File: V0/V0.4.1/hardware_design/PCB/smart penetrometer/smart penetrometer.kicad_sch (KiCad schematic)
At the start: 22 parts, among them J1 Conn_01x02_Female, J2 XLR3_Switched, J3 Conn_01x07_Female, U1 ADS1120-PW, U2 DS3231M, U3 4023, U4 ADS1115IDGS

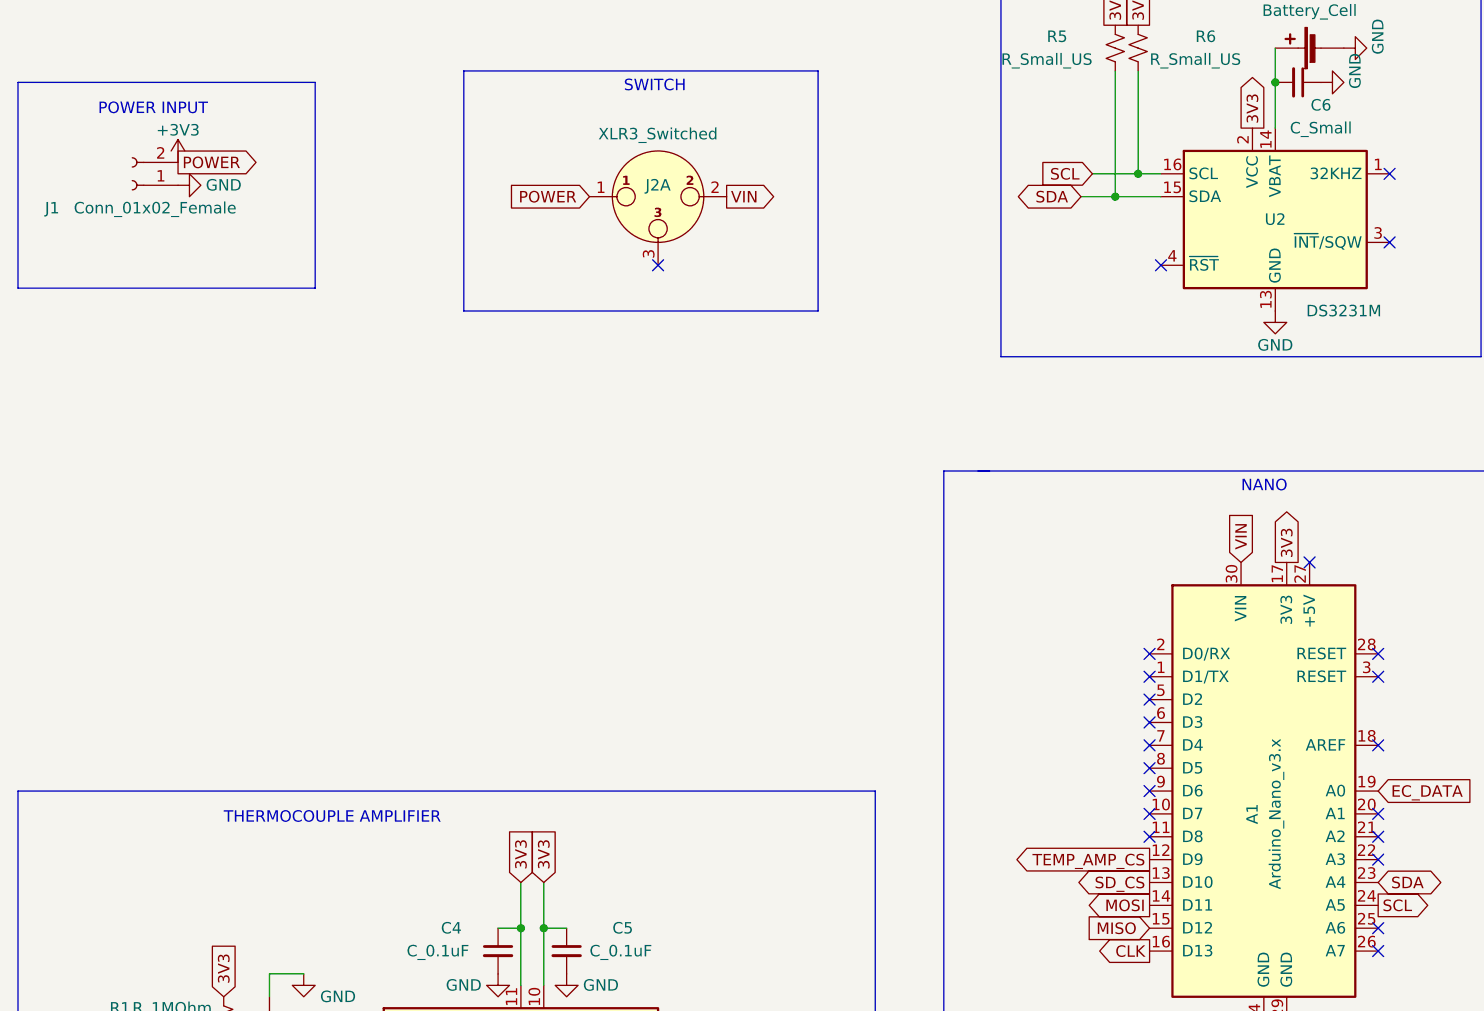
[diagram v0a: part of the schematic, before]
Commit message: PCB V0.4.1 UPDATE
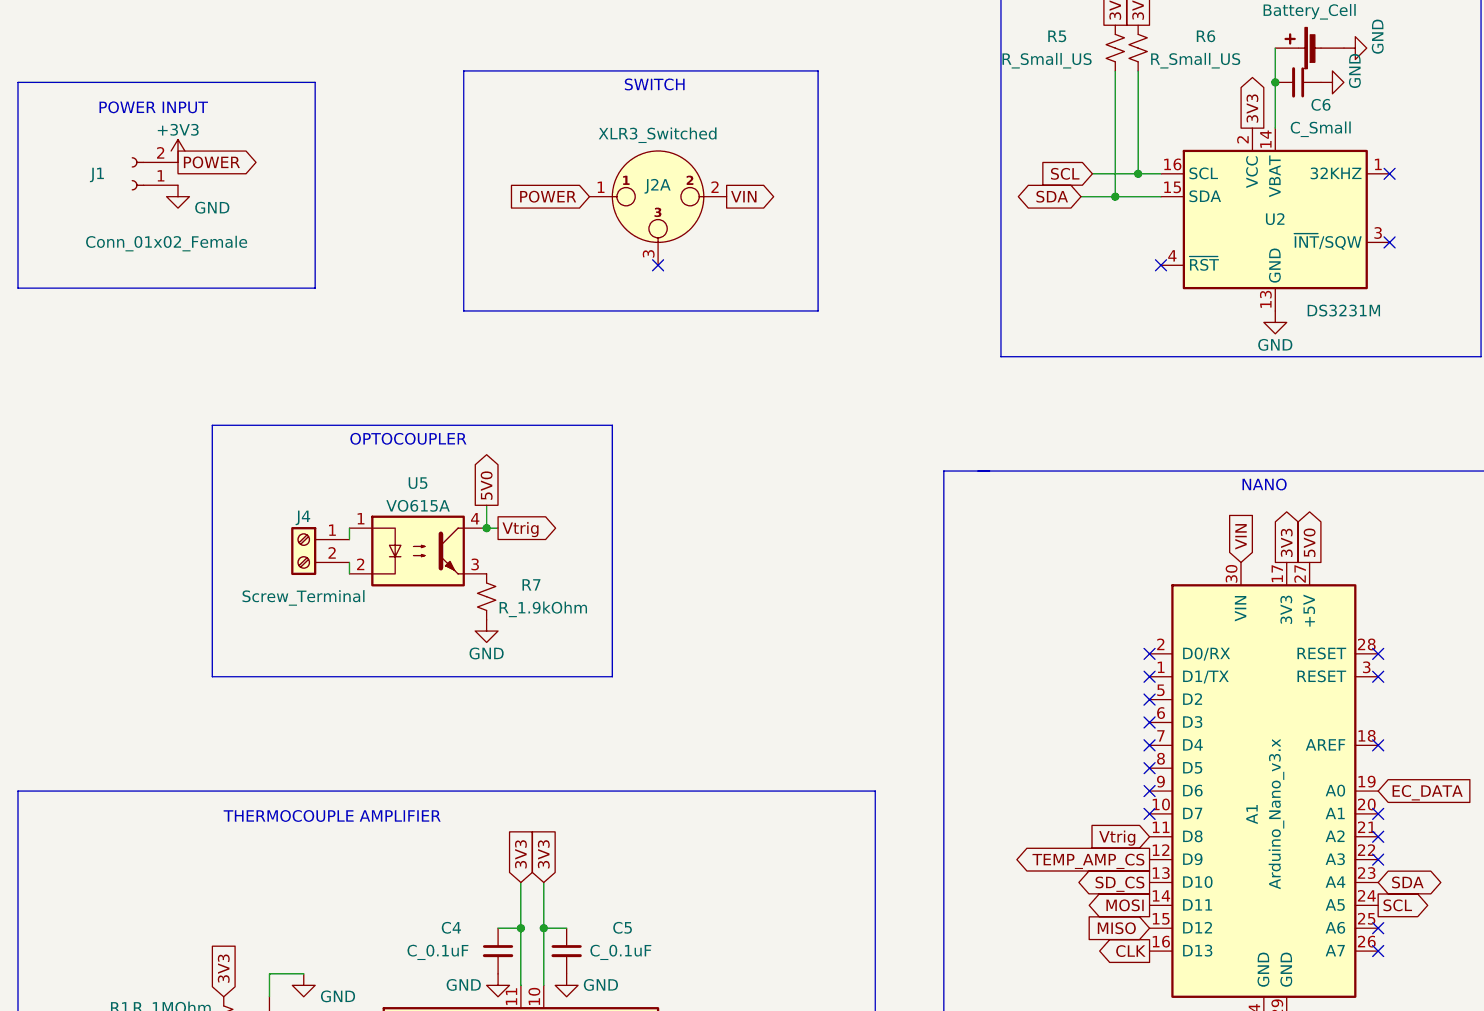
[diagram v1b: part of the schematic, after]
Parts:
- added J4: Screw_Terminal, TerminalBlock:TerminalBlock_bornier-2_P5.08mm, symbol Connector:Screw_Terminal_01x02
- added R7: R_1.9kOhm, Resistor_SMD:R_1206_3216Metric, symbol Device:R_Small_US
- added U5: VO615A, footprints:Vishay_VOS615A, symbol Isolator:VO615A
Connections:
- net GND: now also R7.2
- net 5V0: now reaches A1.11 (D8)
- net 5V0: now also A1.27 (+5V), U5.4
- new net: R7.1, U5.3
- new net: J4.1 (Pin_1), U5.1
- new net: J4.2 (Pin_2), U5.2
- no-connect marks 31 -> 29
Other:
- note added: "OPTOCOUPLER"
